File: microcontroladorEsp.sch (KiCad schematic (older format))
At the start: 37 parts, among them J201 USB_B_Micro, J202 Conn_01x02, J203 Conn_01x02, Q201 S8050, Q202 S8050, Q203 2N7002, Q204 2N7002, SW201 SW_Push, SW202 SW_Push, U201 CP2102N-A01-GQFN28, U202 ESP32-WROOM-32D

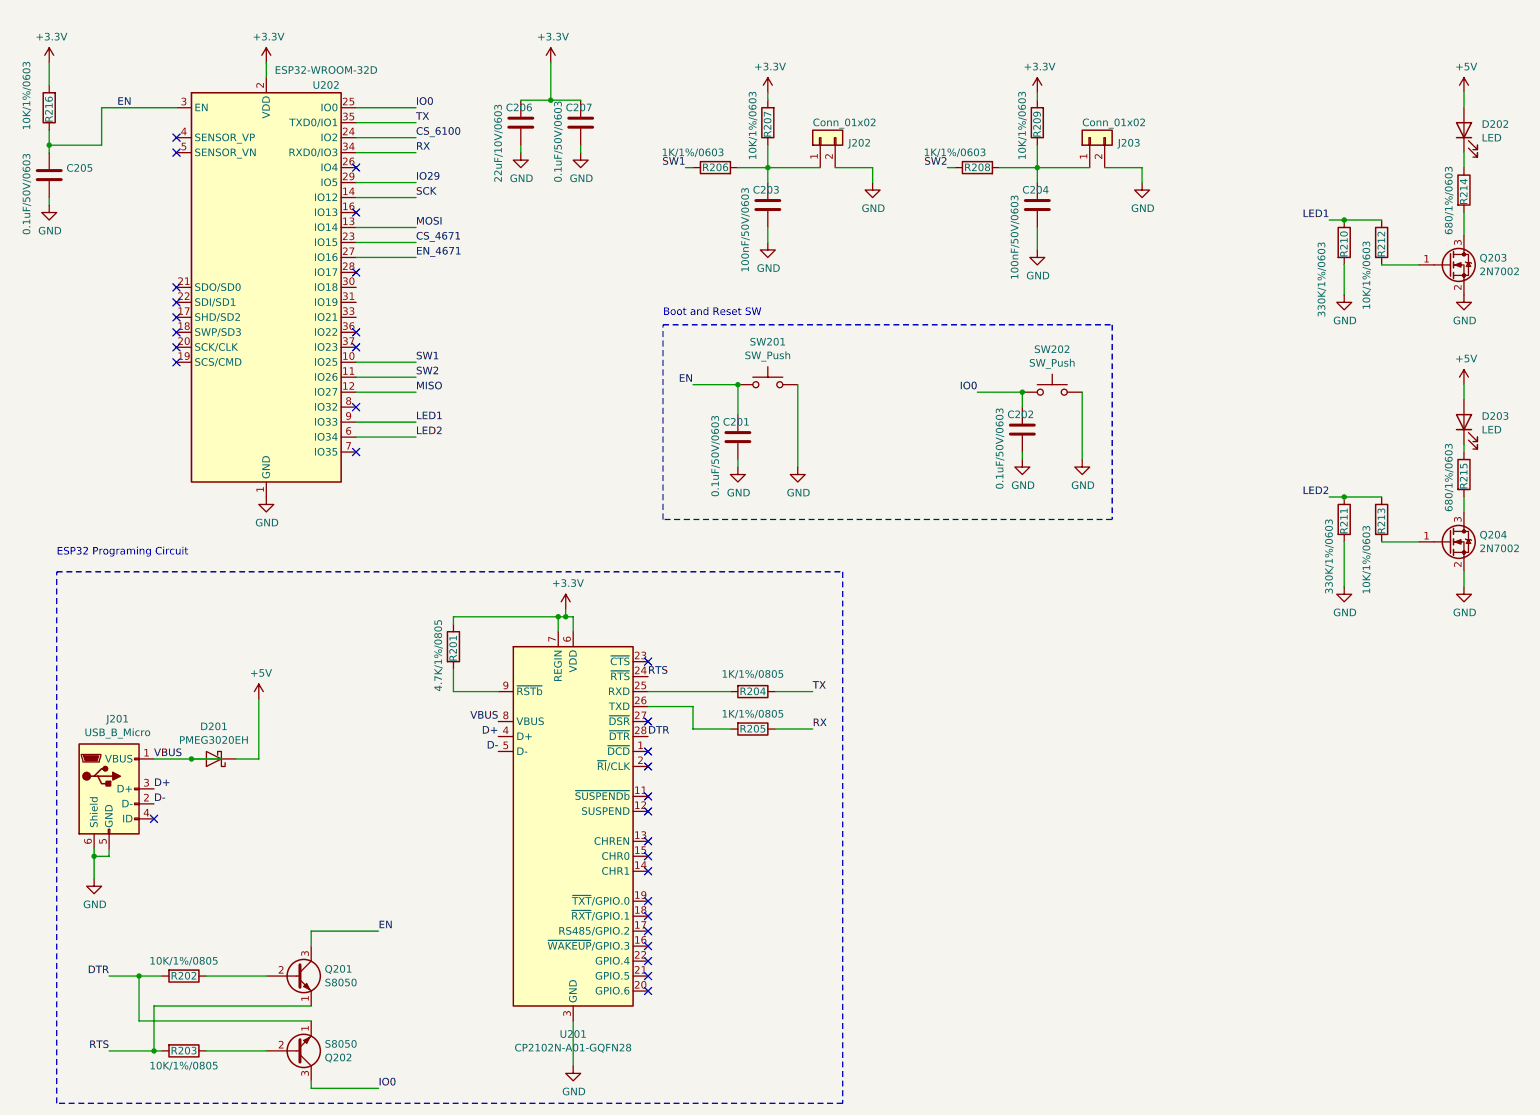
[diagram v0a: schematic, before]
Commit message: ultima actualizacion antes de iniciar el ruteado, diseño verificado
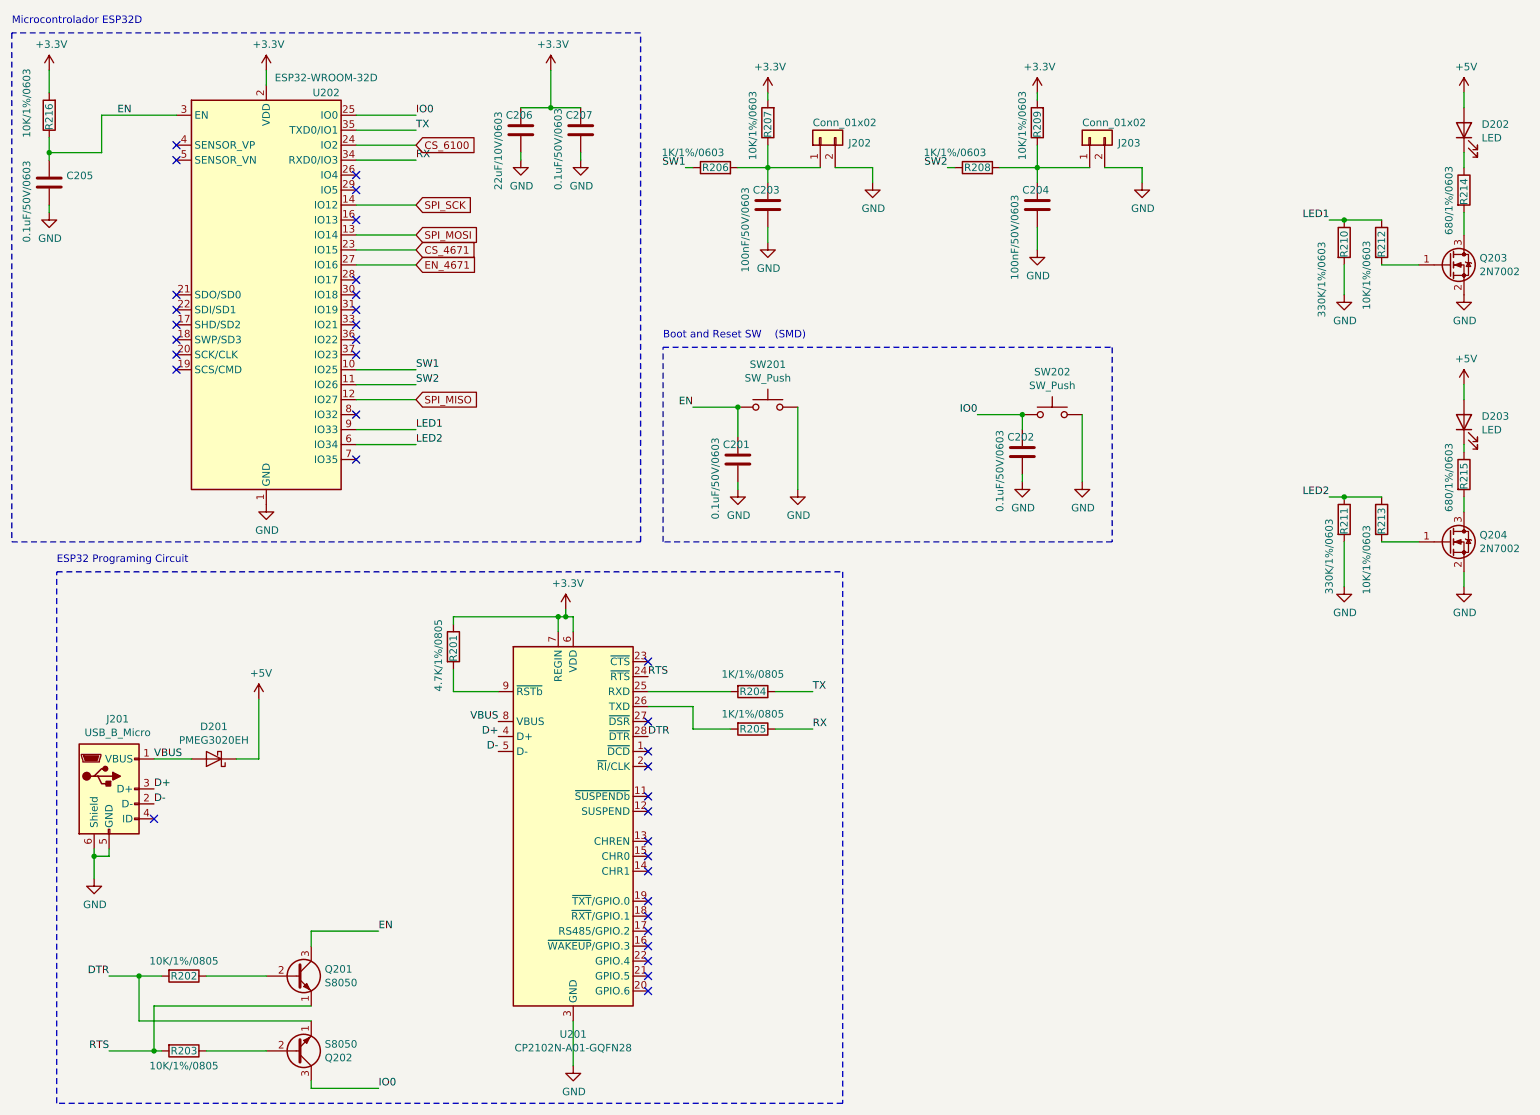
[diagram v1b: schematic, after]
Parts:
- D202, D203: footprint (none) -> LED_SMD:LED_0805_2012Metric
- SW201, SW202: footprint (none) -> KSR223GLFG:KSR223GLFG
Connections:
- net IO29: no longer names the net of U202.29 (IO5)
- net MISO renamed SPI_MISO
- net MOSI renamed SPI_MOSI
- net SCK renamed SPI_SCK
- no-connect marks 32 -> 36
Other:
- note added: "Boot and Reset SW (SMD)"
- note added: "Microcontrolador ESP32D"
- note removed: "Boot and Reset SW"
- moved on the sheet: C201, C202, C205, C206, C207, R216, SW201, SW202, U202
